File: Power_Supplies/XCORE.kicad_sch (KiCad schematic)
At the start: 7 parts, among them U10 XU316-1024-TQ128-I24, U11 W25Q64JVSSIQ (FLASH MEMORY), X1 FA-238 24.0000MB-C0 (CRYSTAL)

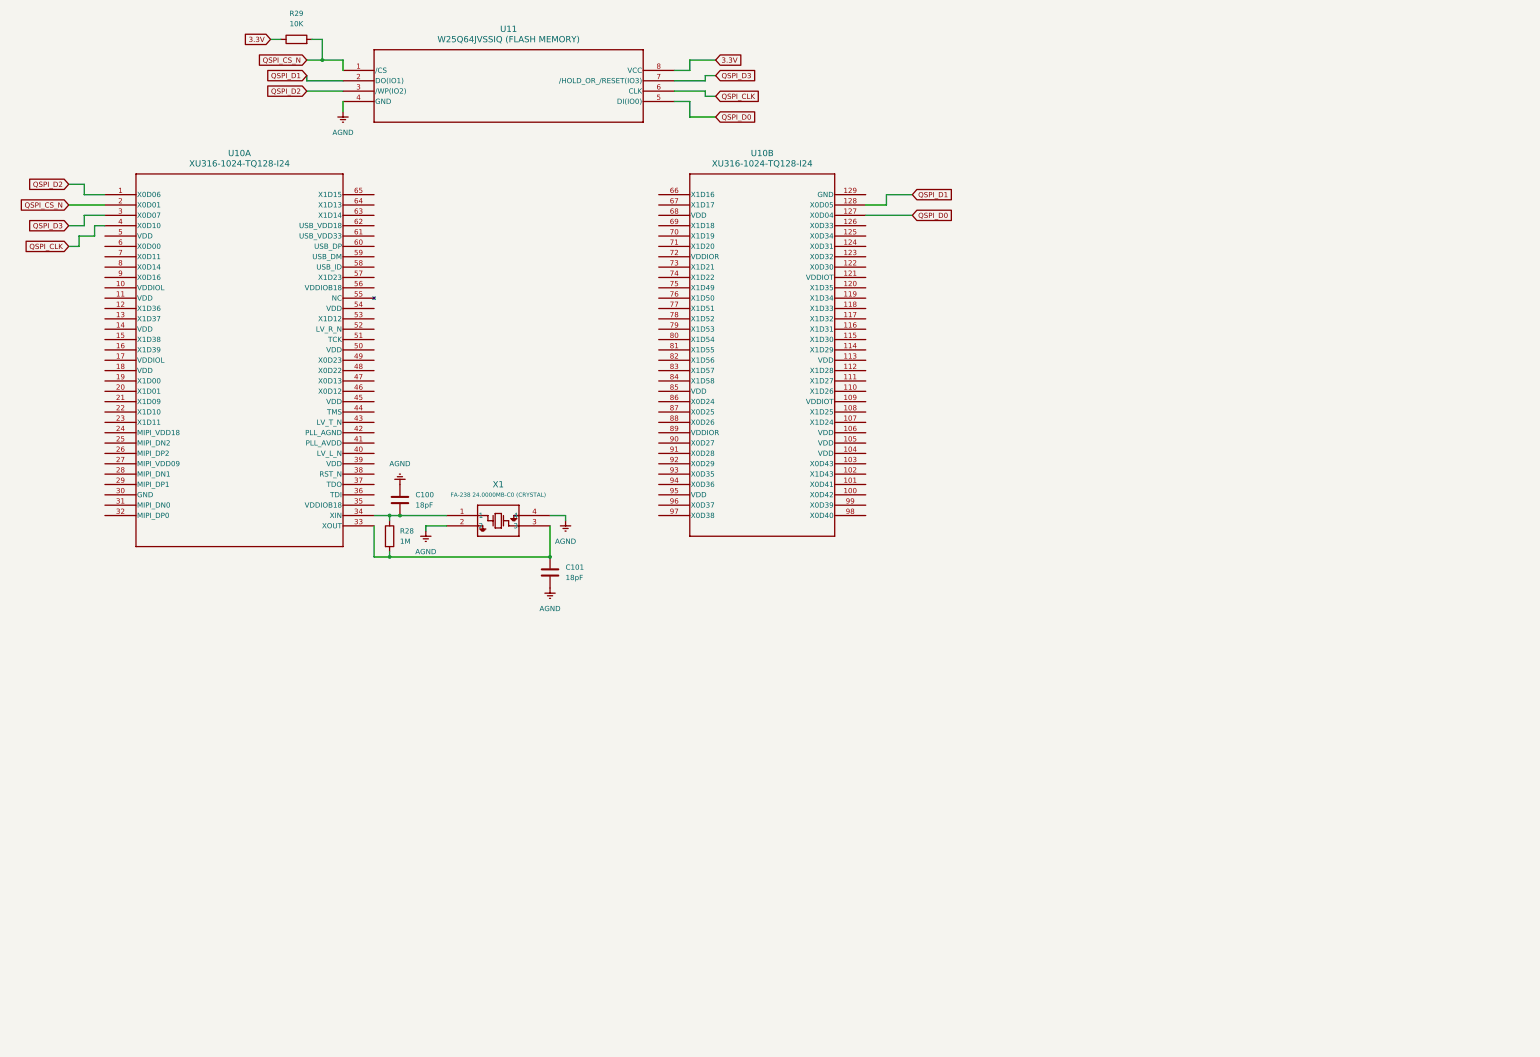
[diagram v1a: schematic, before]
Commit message: Finished HiZ Inputs
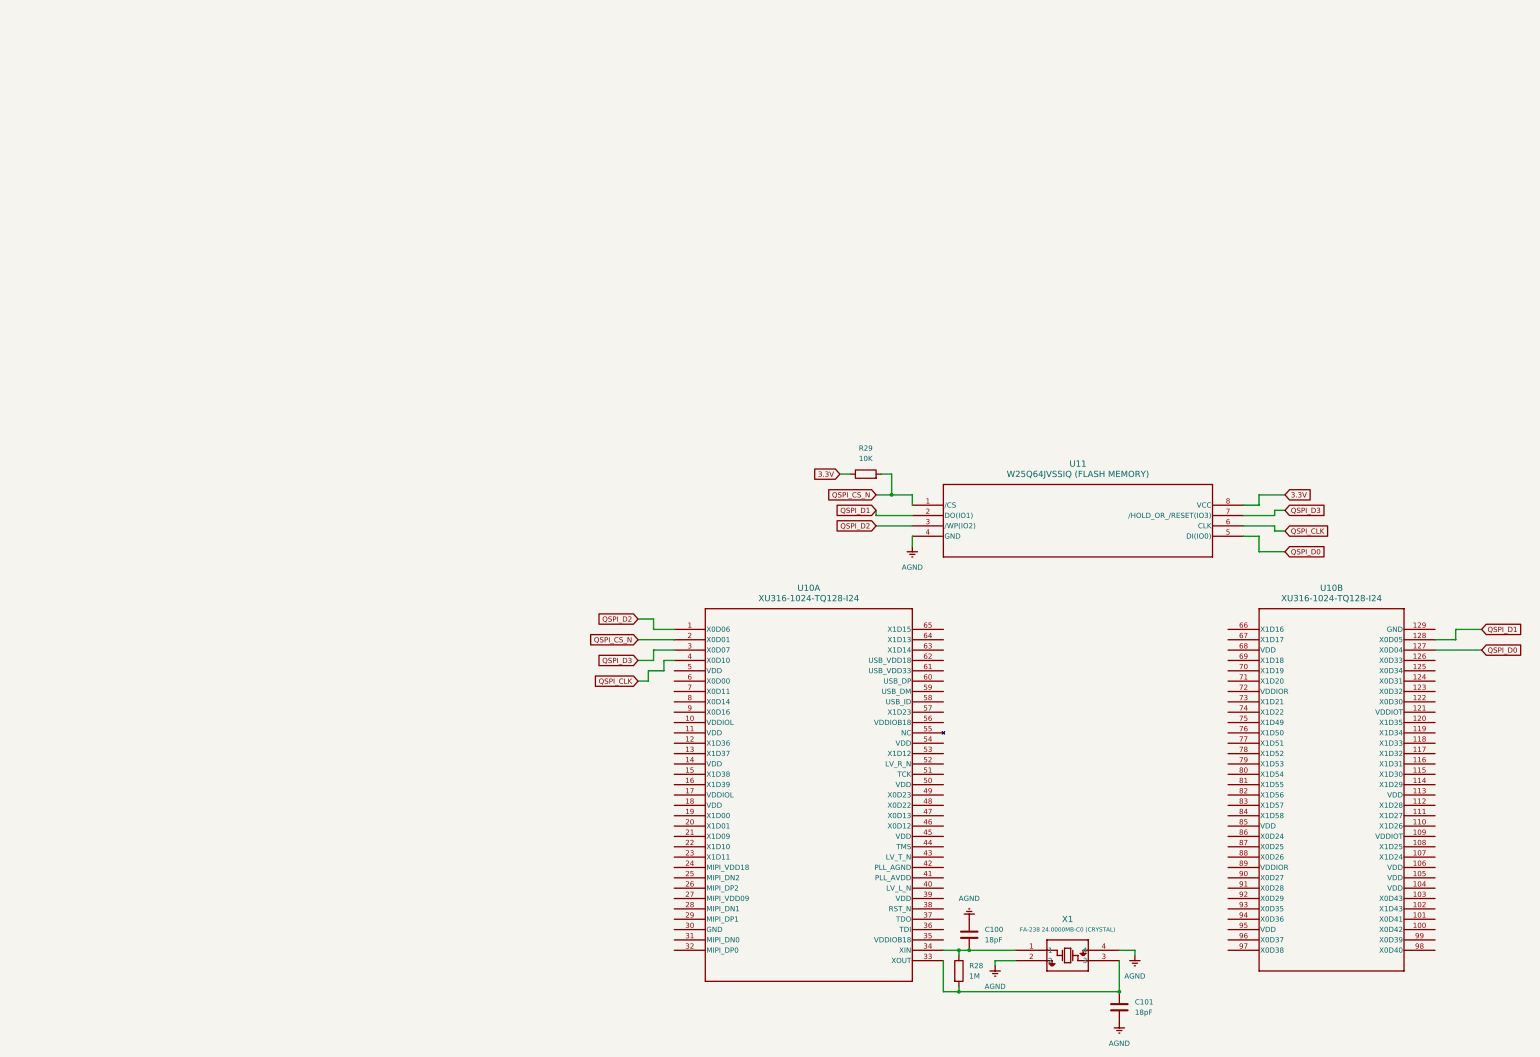
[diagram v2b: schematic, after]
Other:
- moved on the sheet: C100, C101, R28, R29, U10A, U10B, U11, X1
